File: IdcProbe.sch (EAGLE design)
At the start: 79 parts, among them IC1 TL074D, J1 PSL2G, P1 BANANA_SOCKETVERTICAL, P2 BANANA_SOCKETVERTICAL, Q1 PMV45EN, U1 NCP361MUTBG, U2 TPS65131RGET, U3 CMS3005, X1 R141426

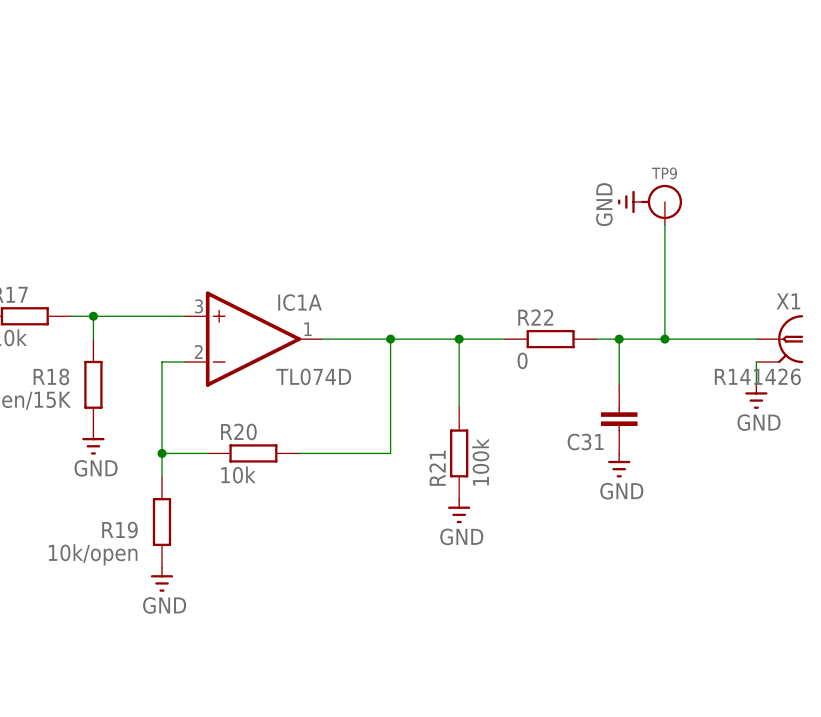
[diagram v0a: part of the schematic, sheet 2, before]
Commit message: Accumulated fixes during testing for version 1.2
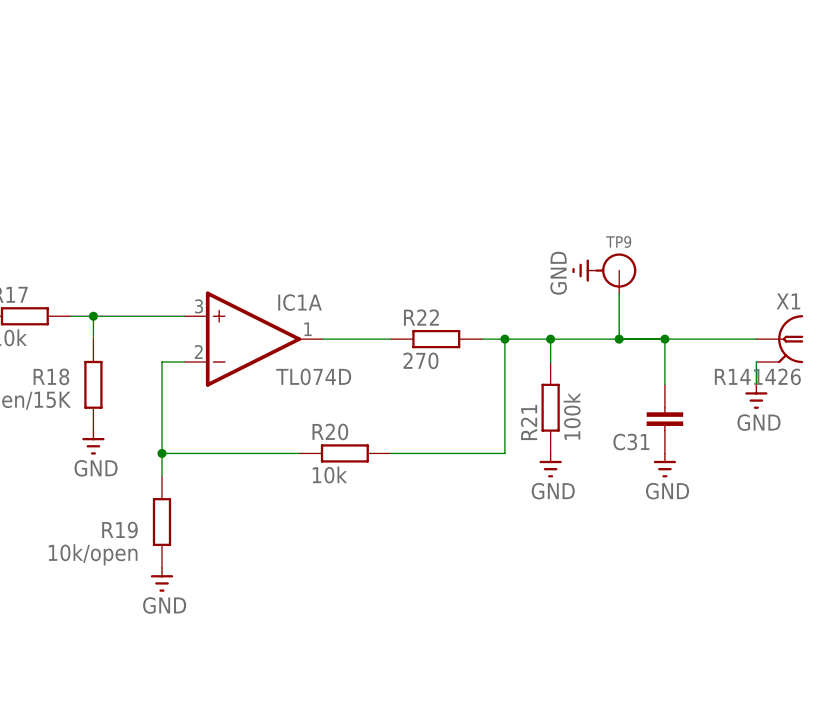
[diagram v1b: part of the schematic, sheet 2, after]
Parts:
- R22: value 0 -> 270
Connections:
- removed net N$12: C31.2, R22.2, TP9.P$1, X1.1
- new net N$22: IC1A.OUT, R22.1
- net N$11: now also C31.2, R22.2, TP9.P$1, X1.1; no longer IC1A.OUT, R22.1
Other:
- moved on the sheet: C31, R20, R21, R22, TP9
